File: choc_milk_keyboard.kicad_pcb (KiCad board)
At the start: 2 copper layers, 20 x 38 mm, 6 parts, among them J1 Conn_01x02_Female, SW1 SW_PUSH, SW2 SW_PUSH, U1 ProMicro

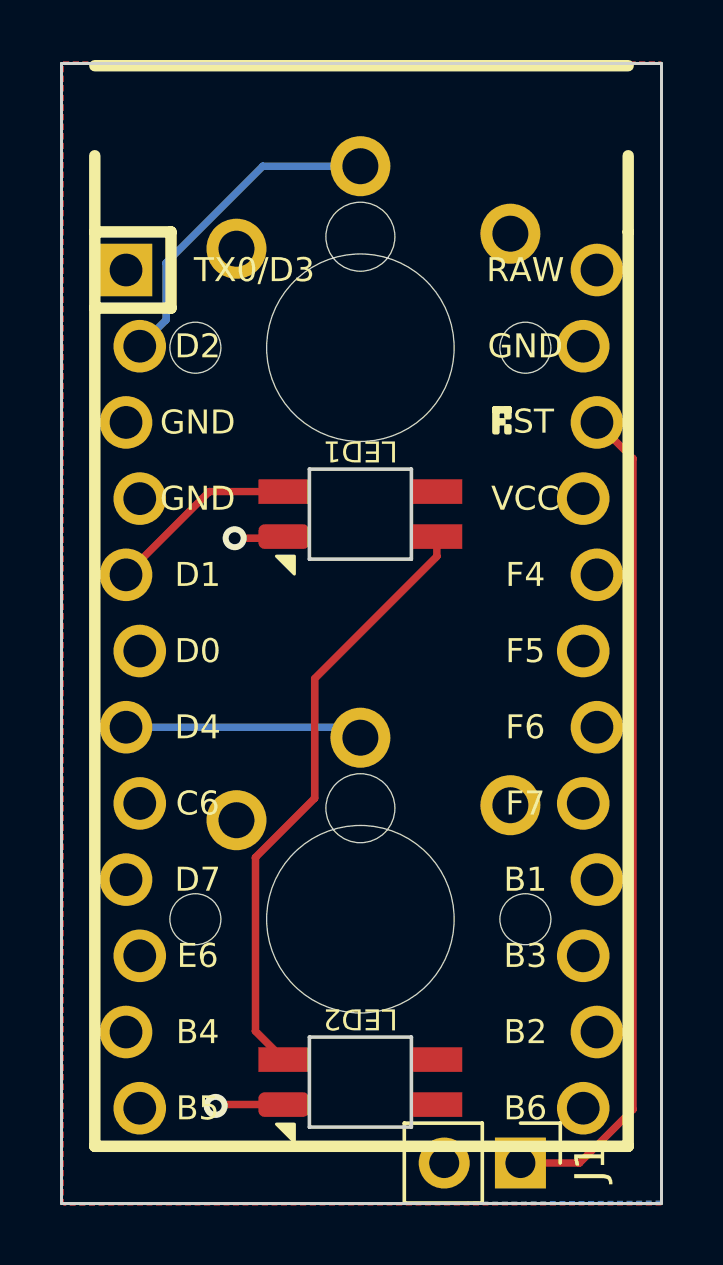
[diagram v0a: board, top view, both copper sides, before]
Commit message: Added 3d models, flipped pro micro
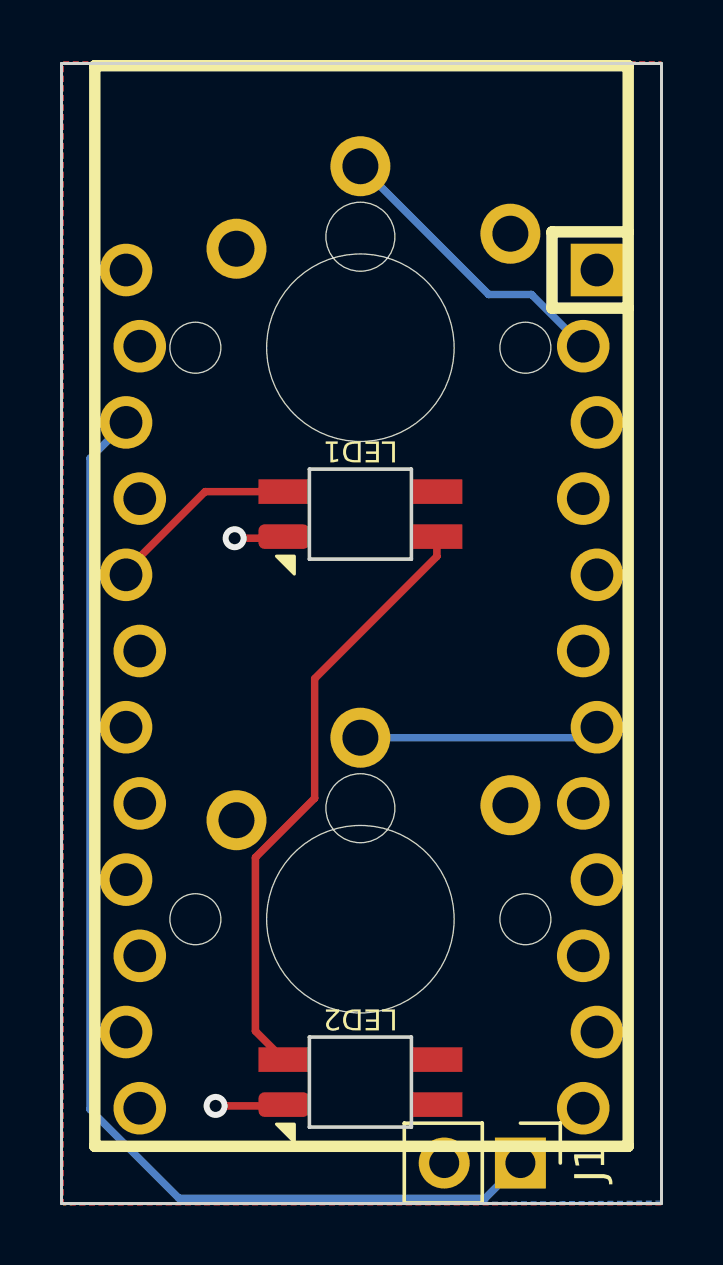
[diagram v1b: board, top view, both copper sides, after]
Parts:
- SW1, SW2: footprint ergodonk_kicad_library:Low-Profile-Choc-MX -> ergodonk_kicad_library:Low-Profile-Choc-MX_no_text
- U1: moved to B.Cu
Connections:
- LED1 pad 4: Net-(U1-Pad5) -> unconnected-(LED1-Pad4)
- U1 pad 20: unconnected-(U1-Pad20) -> unconnected-(LED1-Pad4)
- U1 pad 5: Net-(U1-Pad5) -> unconnected-(U1-Pad5)
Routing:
- net Net-(J1-Pad1): track 27.9 -> 39.5 mm
- net unconnected-(LED1-Pad4): track 0.00 -> 6.54 mm
- net Net-(U1-Pad5): track 6.41 -> 0.00 mm
- net Net-(SW1-Pad1): track 11.0 -> 9.91 mm
